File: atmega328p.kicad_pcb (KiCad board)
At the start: 2 copper layers, 68.6 x 53.3 mm, 40 parts, among them CON1 Micro USB, CON2 AVR-ISP-6, IC1 DS3231M_SO16, IC2 LD1117, IC3 ATMEGA328P-TQFP32, M1 D1, P5 CONN_1, P6 CONN_1, P7 CONN_1, P8 CONN_1, SW1 RESET, X1 16 MHz

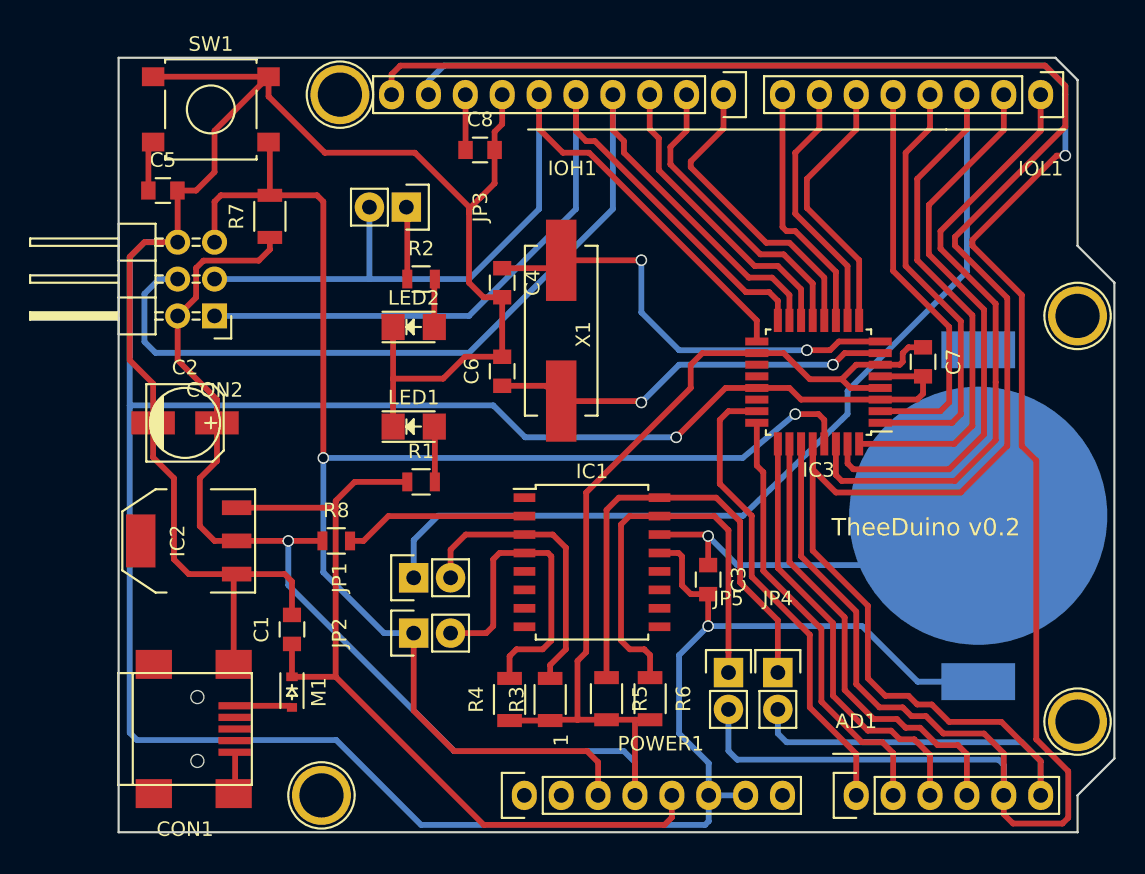
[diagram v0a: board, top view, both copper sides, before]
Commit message: Updated drill files
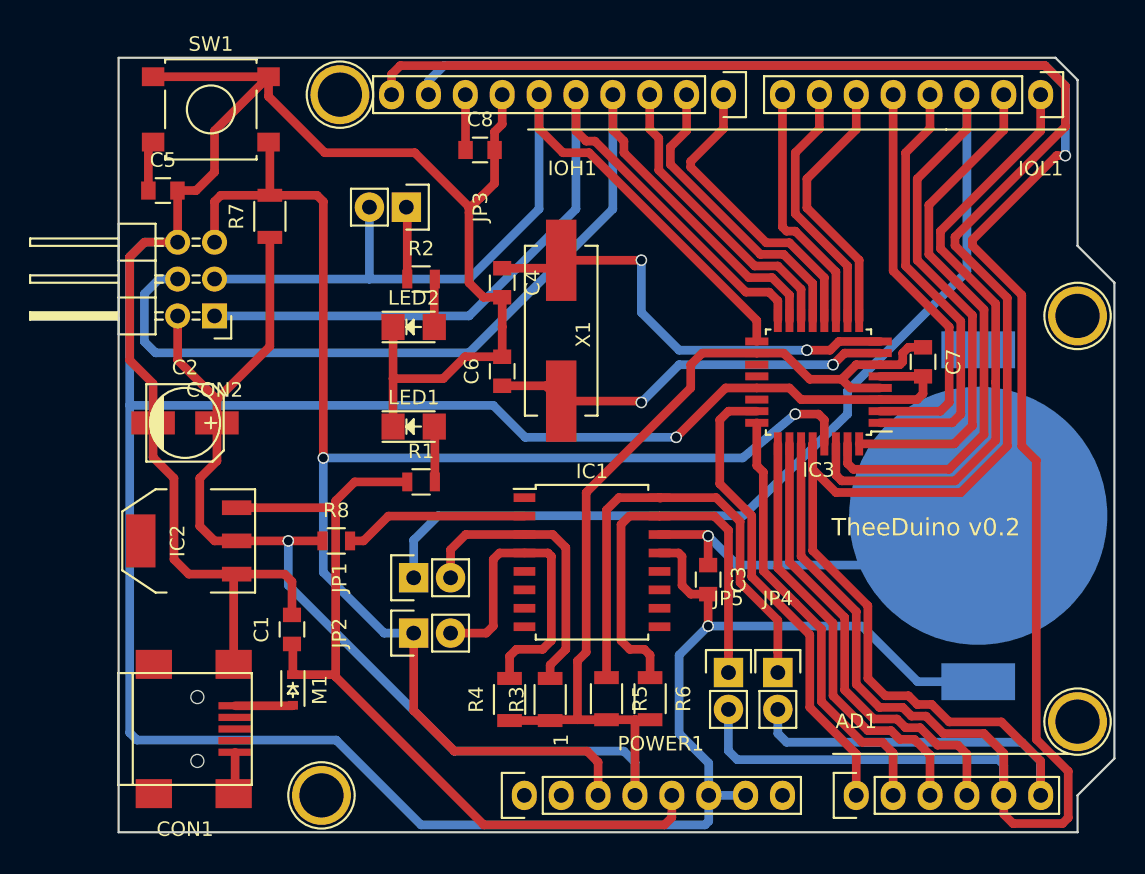
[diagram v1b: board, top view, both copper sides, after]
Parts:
- moved M1 0.16 mm to (123.0, 116.6)
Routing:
- net +3V3: track 134.0 -> 136.1 mm
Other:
- net class Default: clearance 0.2 -> 0.1; trace_width 0.4 -> 0.6
- rule trace_clearance: 0.2 -> 0.1
- rule trace_min: 0.4 -> 0.6
